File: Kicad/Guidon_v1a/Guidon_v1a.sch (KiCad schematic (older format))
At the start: 29 parts, among them IC1 MCP2562, IC2 R-785.0-0.5, K1 ALIM, K2 BUS CAN, K3 INTER., K4 OLED

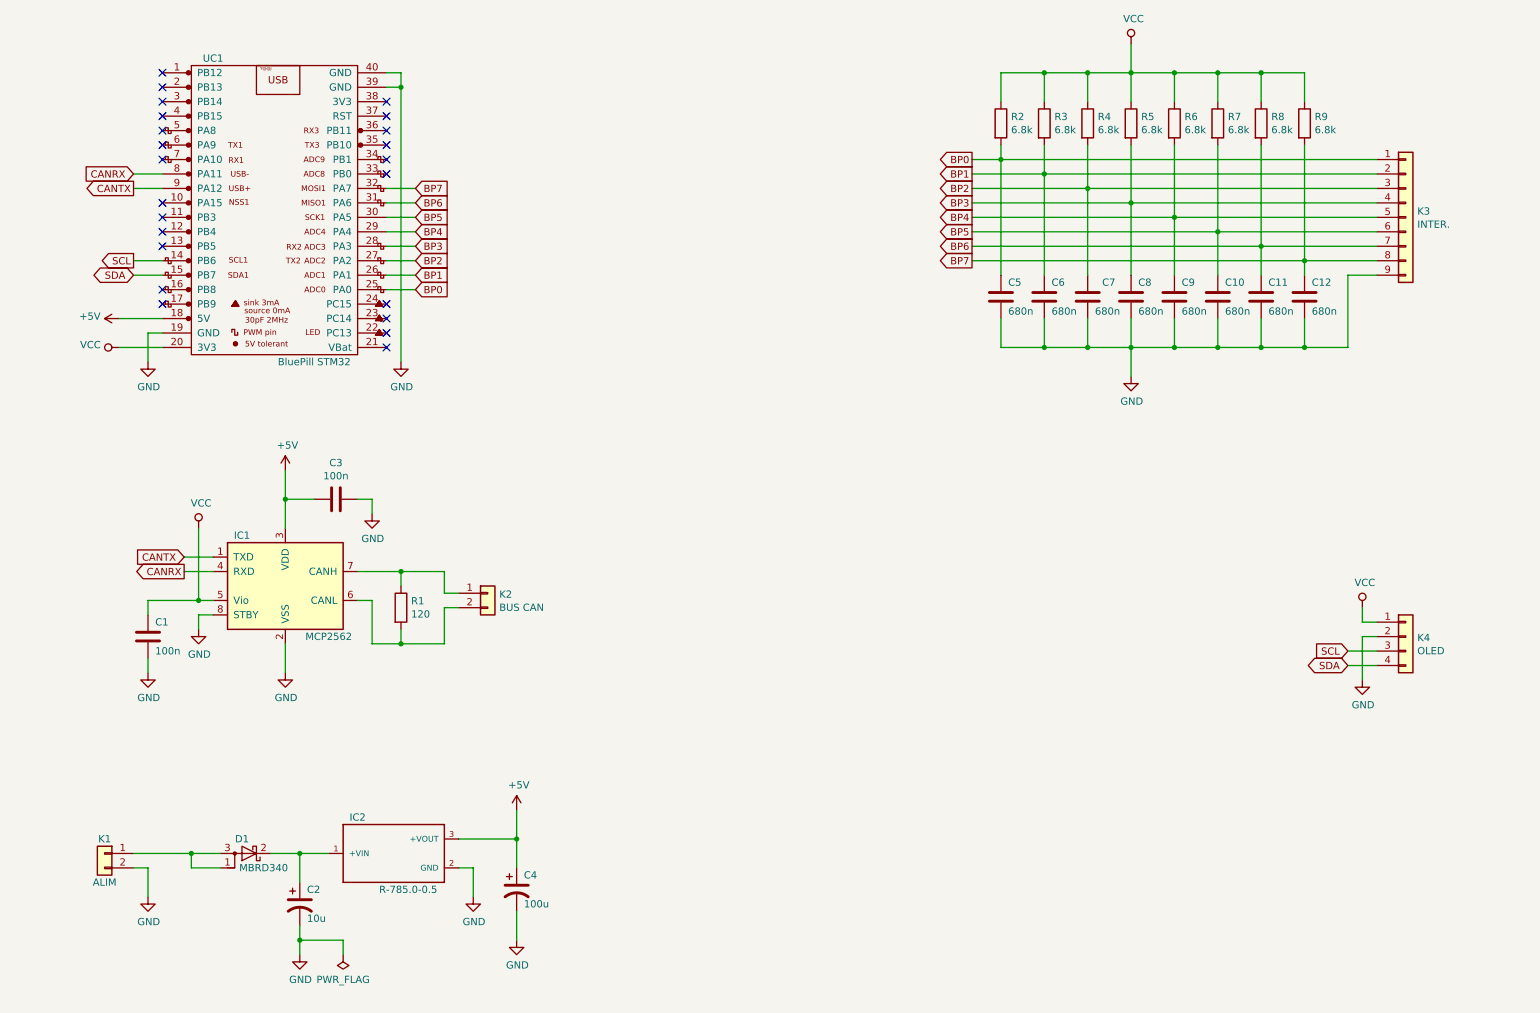
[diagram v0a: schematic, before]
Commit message: Update
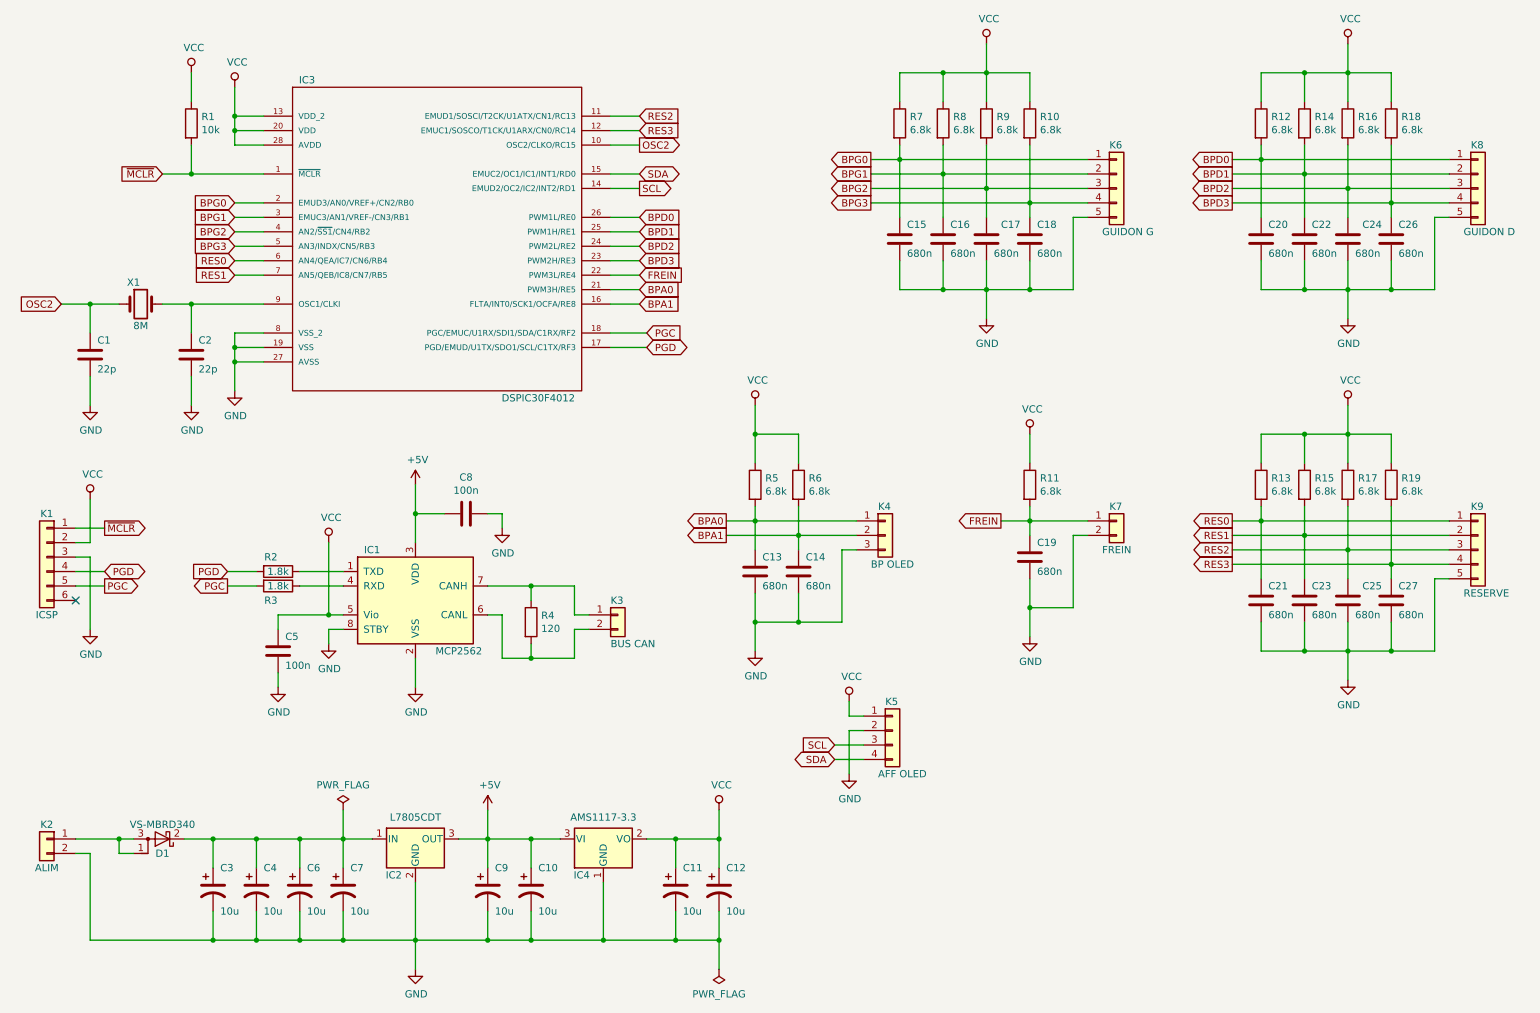
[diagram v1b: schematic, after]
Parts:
- removed C10, C11, C12, C9: 680n, symbol Device:C
- removed C2: 10u, symbol Device:CP1
- removed IC2: R-785.0-0.5, RECOM_R-785.0-0.5, symbol R-785.0-0.5:R-785.0-0.5
- removed K1: ALIM, symbol Connector_Generic:Conn_01x02
- removed K3: INTER., symbol Connector_Generic:Conn_01x09
- removed R7, R8, R9: 6.8k, symbol Device:R
- removed UC1: BluePill STM32, symbol YAAJ_STM32:BluePill_1
- added C1, C2: 22p, symbol Device:C
- added C10, C11, C12, C3, C6, C7, C9: 10u, symbol Device:CP1
- added C13, C14, C19, C20, C21, C22, C23, C24, C25, C26, C27: 680n, symbol Device:C
- added IC2: L7805CDT, symbol Regulator_Linear:L7805
- added IC3: DSPIC30F4012, SOIC127P1030X265-28N, symbol DSPIC30F4012-20I_SO:DSPIC30F4012-20I_SO
- added IC4: AMS1117-3.3, symbol Regulator_Linear:LM1117-3.3
- added K1: ICSP, symbol Connector_Generic:Conn_01x06
- added K2: ALIM, symbol Connector_Generic:Conn_01x02
- added K4: BP OLED, symbol Connector_Generic:Conn_01x03
- added K6: GUIDON G, symbol Connector_Generic:Conn_01x05
- added K7: FREIN, symbol Connector_Generic:Conn_01x02
- added K8: GUIDON D, symbol Connector_Generic:Conn_01x05
- added K9: RESERVE, symbol Connector_Generic:Conn_01x05
- added R1: 10k, symbol Device:R
- added R11, R12, R13, R14, R15, R16, R17, R18, R19, R5: 6.8k, symbol Device:R
- added R2, R3: 1.8k, symbol Device:R
- added X1: 8M, symbol Device:Crystal
- C4: value 100u -> 10u
- D1: value MBRD340 -> VS-MBRD340
- K5: renamed from K4; value OLED -> AFF OLED
- renumbered C5 to C15, C6 to C16, C7 to C17, C8 to C18, C1 to C5, C3 to C8, K2 to K3, R5 to R10, R1 to R4, R2 to R7, R3 to R8, R4 to R9
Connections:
- net +5V: now also C10.1, C9.1, IC2.3 (OUT), IC4.3 (VI); no longer C4.1
- net GND: now also C1.2, C10.2, C11.2, C12.2, C13.2, C14.2, C19.2, C2.2, C20.2, C21.2, C22.2, C23.2, C24.2, C25.2, C26.2, C27.2, C3.2, C6.2, C7.2, C9.2, IC2.2 (GND), IC3.19 (VSS), IC3.27 (AVSS), IC3.8 (VSS_2), IC4.1 (GND), K1.3 (Pin_3), K2.2 (Pin_2), K4.3 (Pin_3), K6.5 (Pin_5), K7.2 (Pin_2), K8.5 (Pin_5), K9.5 (Pin_5)
- net SCL: now also IC3.14 (EMUD2/OC2/IC2/INT2/RD1)
- net SDA: now also IC3.15 (EMUC2/OC1/IC1/INT1/RD0)
- net VCC: now also C11.1, C12.1, IC3.13 (VDD_2), IC3.20 (VDD), IC3.28 (AVDD), IC4.2 (VO), K1.2 (Pin_2), R1.1, R11.1, R12.1, R13.1, R14.1, R15.1, R16.1, R17.1, R18.1, R19.1, R5.1
- net at D1.2 (K): now also C4.1, C3.1, C6.1, C7.1, IC2.1 (IN)
- net at D1.1 (A), D1.3 (A): now also K2.1 (Pin_1)
- net BP0 renamed BPG0
- net BPG0: now also IC3.2 (EMUD3/AN0/VREF+/CN2/RB0), K6.1 (Pin_1)
- net BP1 renamed BPG1
- net BPG1: now also IC3.3 (EMUC3/AN1/VREF-/CN3/RB1), K6.2 (Pin_2)
- net BP2 renamed BPG2
- net BPG2: now also IC3.4 (AN2/~SS1~/CN4/RB2), K6.3 (Pin_3)
- net BP3 renamed BPG3
- net BPG3: now also IC3.5 (AN3/INDX/CN5/RB3), K6.4 (Pin_4)
- net BP4 renamed BPA1
- net BPA1: now also C14.1, IC3.16 (FLTA/INT0/SCK1/OCFA/RE8), K4.2 (Pin_2)
- net CANRX: no longer names the net of IC1.4 (RXD)
- net CANRX: now also R3.1
- net CANTX: no longer names the net of IC1.1 (TXD)
- net CANTX: now also R2.1
- new net: C2.1, IC3.9 (OSC1/CLKI), X1.2
- new net BPA0: C13.1, IC3.21 (PWM3H/RE5), K4.1 (Pin_1), R5.2
- new net BPD0: C20.1, IC3.26 (PWM1L/RE0), K8.1 (Pin_1), R12.2
- new net BPD1: C22.1, IC3.25 (PWM1H/RE1), K8.2 (Pin_2), R14.2
- new net BPD2: C24.1, IC3.24 (PWM2L/RE2), K8.3 (Pin_3), R16.2
- new net BPD3: C26.1, IC3.23 (PWM2H/RE3), K8.4 (Pin_4), R18.2
- new net FREIN: C19.1, IC3.22 (PWM3L/RE4), K7.1 (Pin_1), R11.2
- new net OSC2: C1.1, IC3.10 (OSC2/CLKO/RC15), X1.1
- new net PGC: IC3.18 (PGC/EMUC/U1RX/SDI1/SDA/C1RX/RF2), K1.5 (Pin_5), R3.2
- new net PGD: IC3.17 (PGD/EMUD/U1TX/SDO1/SCL/C1TX/RF3), K1.4 (Pin_4), R2.2
- new net RES0: C21.1, IC3.6 (AN4/QEA/IC7/CN6/RB4), K9.1 (Pin_1), R13.2
- new net RES1: C23.1, IC3.7 (AN5/QEB/IC8/CN7/RB5), K9.2 (Pin_2), R15.2
- new net RES2: C25.1, IC3.11 (EMUD1/SOSCI/T2CK/U1ATX/CN1/RC13), K9.3 (Pin_3), R17.2
- new net RES3: C27.1, IC3.12 (EMUC1/SOSCO/T1CK/U1ARX/CN0/RC14), K9.4 (Pin_4), R19.2
- new net ~MCLR: IC3.1 (~MCLR), K1.1 (Pin_1), R1.2
- no-connect marks 23 -> 1
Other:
- moved on the sheet: C15, C16, C17, C18, C5, C8, IC1, K3, K5, R10, R4, R7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

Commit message: Update
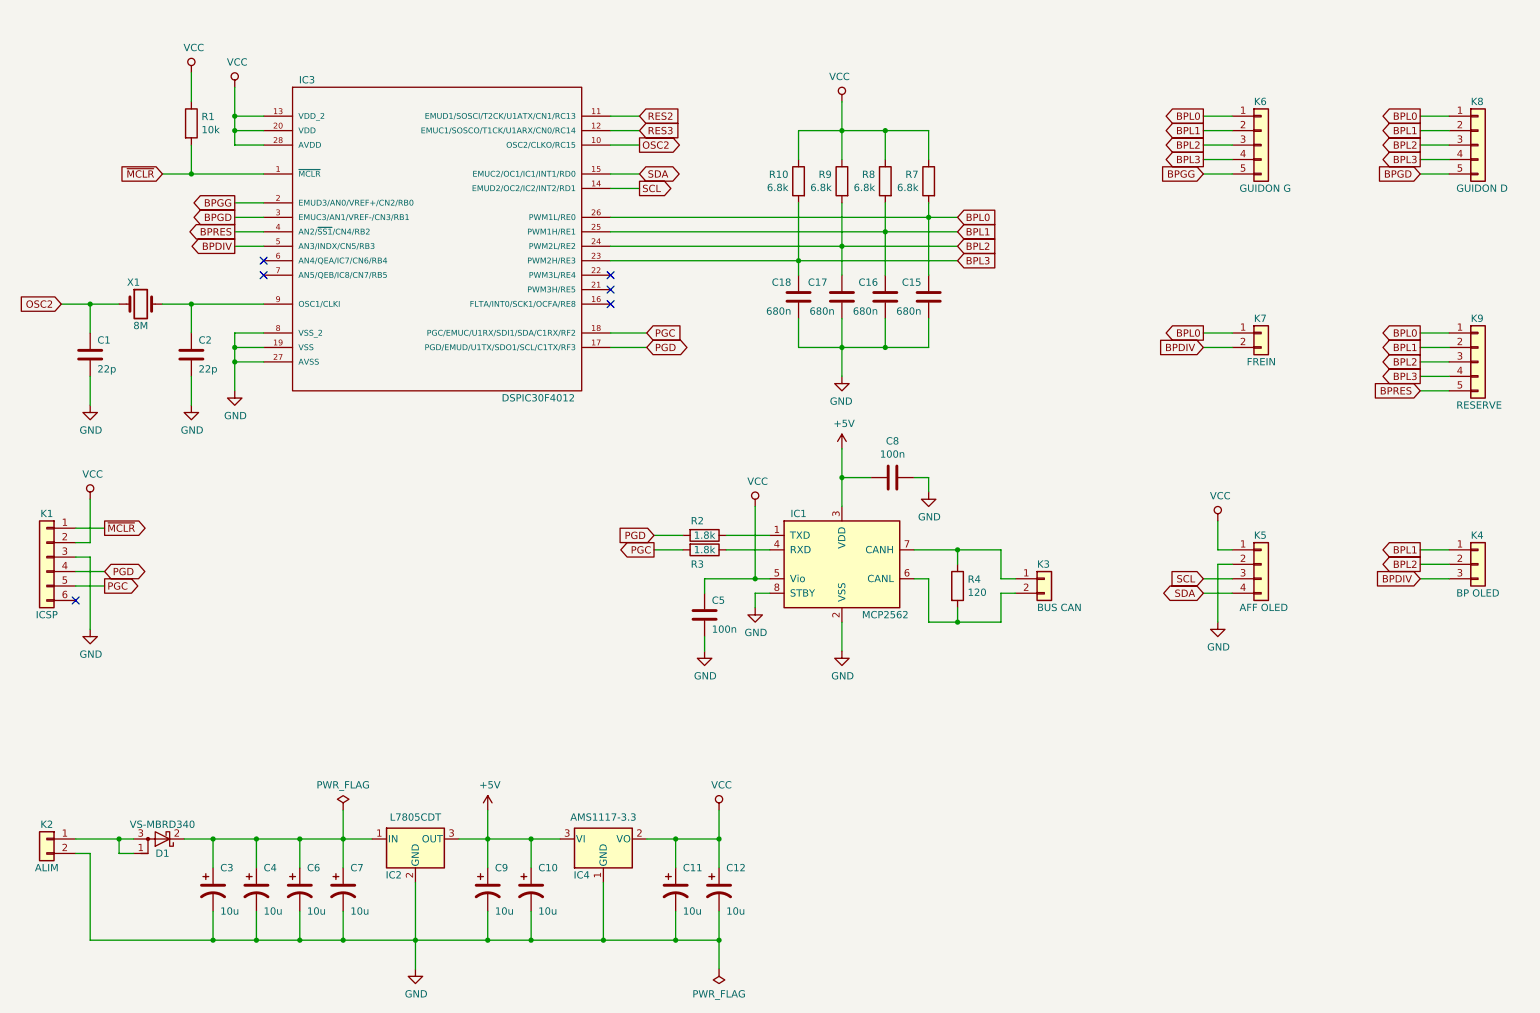
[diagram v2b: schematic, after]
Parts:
- removed C13, C14, C19, C20, C21, C22, C23, C24, C25, C26, C27: 680n, symbol Device:C
- removed R11, R12, R13, R14, R15, R16, R17, R18, R19, R5, R6: 6.8k, symbol Device:R
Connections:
- net GND: no longer K4.3 (Pin_3), K6.5 (Pin_5), K7.2 (Pin_2), K8.5 (Pin_5), K9.5 (Pin_5)
- net RES2: no longer K9.3 (Pin_3)
- net RES3: no longer K9.4 (Pin_4)
- net BPA0: no longer names the net of IC3.21 (PWM3H/RE5)
- net BPA0: no longer K4.1 (Pin_1)
- net BPA1: no longer names the net of IC3.16 (FLTA/INT0/SCK1/OCFA/RE8)
- net BPA1: no longer K4.2 (Pin_2)
- net BPD0 renamed BPL0
- net BPL0: now also C15.1, K6.1 (Pin_1), K7.1 (Pin_1), K9.1 (Pin_1), R7.2
- net BPD1 renamed BPL1
- net BPL1: now also C16.1, K4.1 (Pin_1), K6.2 (Pin_2), K9.2 (Pin_2), R8.2
- net BPD2 renamed BPL2
- net BPL2: now also C17.1, K4.2 (Pin_2), K6.3 (Pin_3), K9.3 (Pin_3), R9.2
- net BPD3 renamed BPL3
- net BPL3: now also C18.1, K6.4 (Pin_4), K9.4 (Pin_4), R10.2
- removed net BPG0: C15.1, IC3.2 (EMUD3/AN0/VREF+/CN2/RB0), K6.1 (Pin_1), R7.2
- removed net BPG1: C16.1, IC3.3 (EMUC3/AN1/VREF-/CN3/RB1), K6.2 (Pin_2), R8.2
- removed net BPG2: C17.1, IC3.4 (AN2/~SS1~/CN4/RB2), K6.3 (Pin_3), R9.2
- removed net BPG3: C18.1, IC3.5 (AN3/INDX/CN5/RB3), K6.4 (Pin_4), R10.2
- net FREIN: no longer names the net of IC3.22 (PWM3L/RE4)
- net FREIN: no longer K7.1 (Pin_1)
- net RES0: no longer names the net of IC3.6 (AN4/QEA/IC7/CN6/RB4)
- net RES0: no longer K9.1 (Pin_1)
- net RES1: no longer names the net of IC3.7 (AN5/QEB/IC8/CN7/RB5)
- net RES1: no longer K9.2 (Pin_2)
- new net BPDIV: IC3.5 (AN3/INDX/CN5/RB3), K4.3 (Pin_3), K7.2 (Pin_2)
- new net BPGD: IC3.3 (EMUC3/AN1/VREF-/CN3/RB1), K8.5 (Pin_5)
- new net BPGG: IC3.2 (EMUD3/AN0/VREF+/CN2/RB0), K6.5 (Pin_5)
- new net BPRES: IC3.4 (AN2/~SS1~/CN4/RB2), K9.5 (Pin_5)
- no-connect marks 1 -> 6
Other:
- moved on the sheet: C15, C16, C17, C18, C5, C8, IC1, K3, K4, K5, K6, K7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
